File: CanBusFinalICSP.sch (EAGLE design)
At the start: 51 parts, among them IC1 PIC16F872P, U1 MCP2515

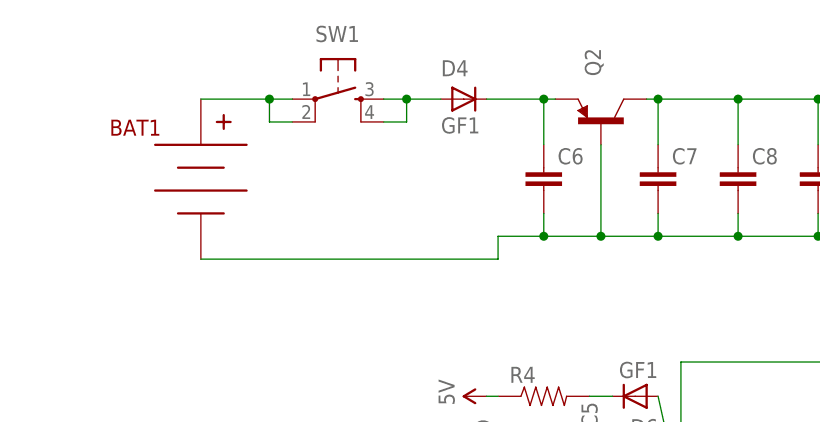
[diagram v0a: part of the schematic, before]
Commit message: Add files via upload
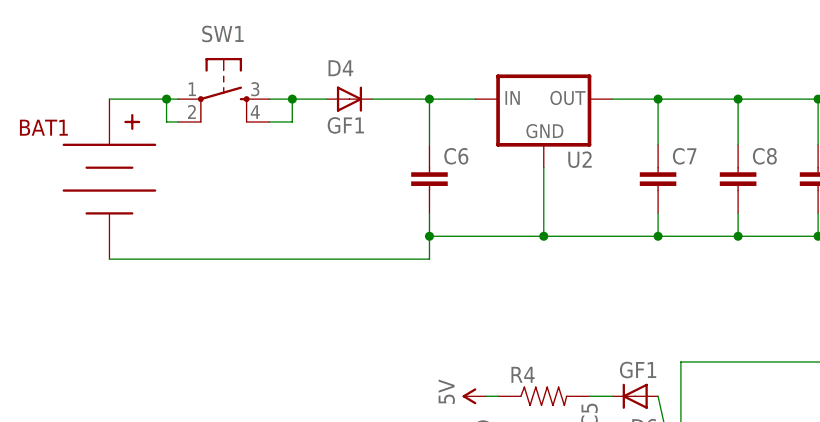
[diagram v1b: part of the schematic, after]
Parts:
- removed Q2: (no value), SparkFun-DiscreteSemi:TRANSISTOR_PNPTO92
- added U2: (no value), SparkFun-PowerIC:V_REG_78XXSIDE
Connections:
- net 5V: now also U2.OUT; no longer Q2.C
- net GND: now also U2.GND; no longer Q2.B
- net N$27: now also U2.IN; no longer Q2.E
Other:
- moved on the sheet: BAT1, C6, D4, SW1
